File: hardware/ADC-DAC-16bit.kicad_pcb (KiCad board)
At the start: 2 copper layers, 21.5 x 21.7 mm, 16 parts, among them J1 CON, J2 DAC, J3 ADC, J4 CH1-, J5 CH2-, U1 AD5667R, U2 MCP3426

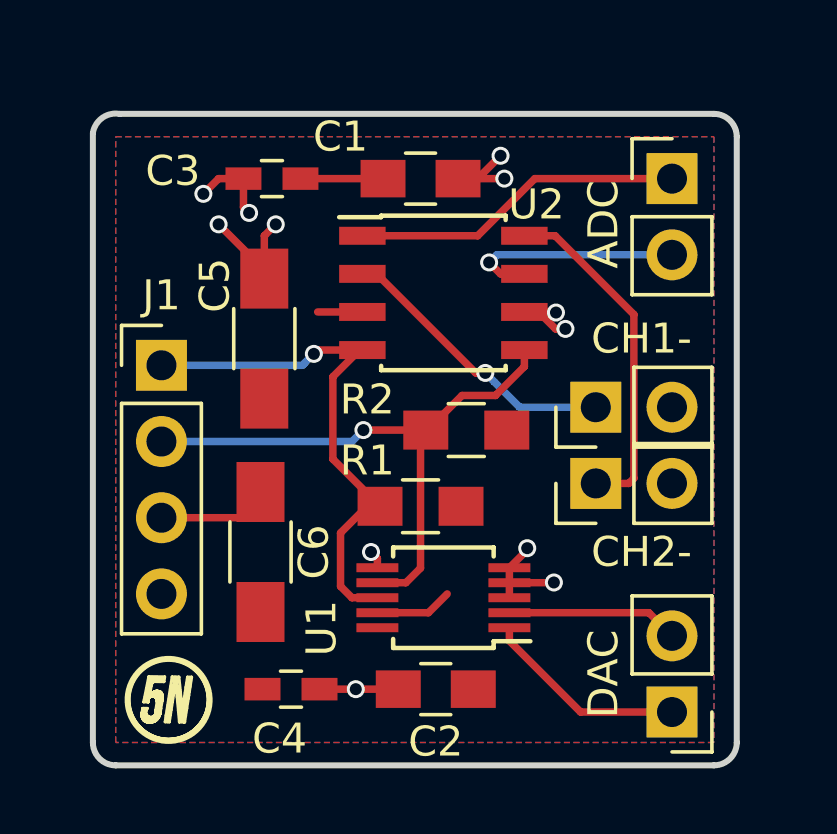
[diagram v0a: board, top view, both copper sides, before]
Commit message: v0.2 update
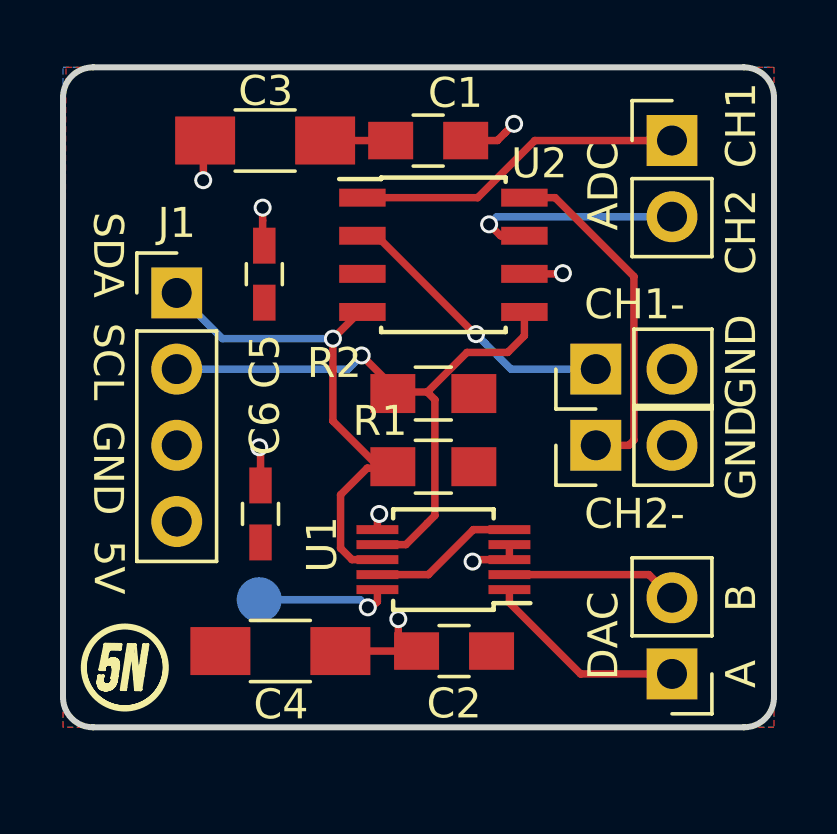
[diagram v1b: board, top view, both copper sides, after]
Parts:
- added TP1: DAC Vref, Measurement_Points:Measurement_Point_Round-SMD-Pad_Small, B.Cu at (138.6, 85.2)
- C3, C4: value 100n -> 10u; footprint Capacitors_SMD:C_0603_HandSoldering -> Capacitors_SMD:C_1206_HandSoldering
- C5, C6: value 10u -> 100n; footprint Capacitors_SMD:C_1206_HandSoldering -> Capacitors_SMD:C_0603_HandSoldering
- moved J1 2.47 mm to (135.9, 74.9)
- moved C5 2.15 mm to (138.8, 74.3)
- moved R2 1.64 mm to (144.4, 78.3)
- moved REF*** 1.42 mm to (143.8, 79.4)
- moved C2 1.41 mm to (145.1, 86.9)
- moved R1 1.39 mm to (144.4, 80.7)
- moved C4 1.32 mm to (139.3, 86.9)
- moved C1 1.29 mm to (144.3, 69.9)
- moved C3 1.29 mm to (138.8, 69.8)
- moved J2 1.27 mm to (152.4, 87.6)
- moved J3 1.27 mm to (152.4, 69.8)
- moved U1 1.27 mm to (144.8, 83.8)
- moved U2 1.27 mm to (144.8, 73.7)
- moved C6 1.27 mm to (138.7, 82.3)
- moved J4 1.27 mm to (149.9, 77.5)
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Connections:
- U1 pad 5: GND -> +5V
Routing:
- net GND: track 24.2 -> 10.6 mm, vias 12 -> 8
- net Net-(TP1-Pad1): track 0.00 -> 4.52 mm, vias 0 -> 1
- net Net-(J1-Pad1): track 18.3 -> 17.0 mm
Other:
- board size 21.5 x 21.7 mm -> 23.7 x 22 mm
- board text added: "2.5v"
- board text added: "5V"
- board text added: "A"
- board text added: "B"
- board text added: "CH1"
- board text added: "CH2"
- board text added: "DAC VREF"
- board text added: "GND"
- board text added: "SCL"
- board text added: "SDA"
- board text added: "v0.2"
